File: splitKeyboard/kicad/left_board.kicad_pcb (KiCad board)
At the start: 2 copper layers, 305 x 136.1 mm, 131 parts

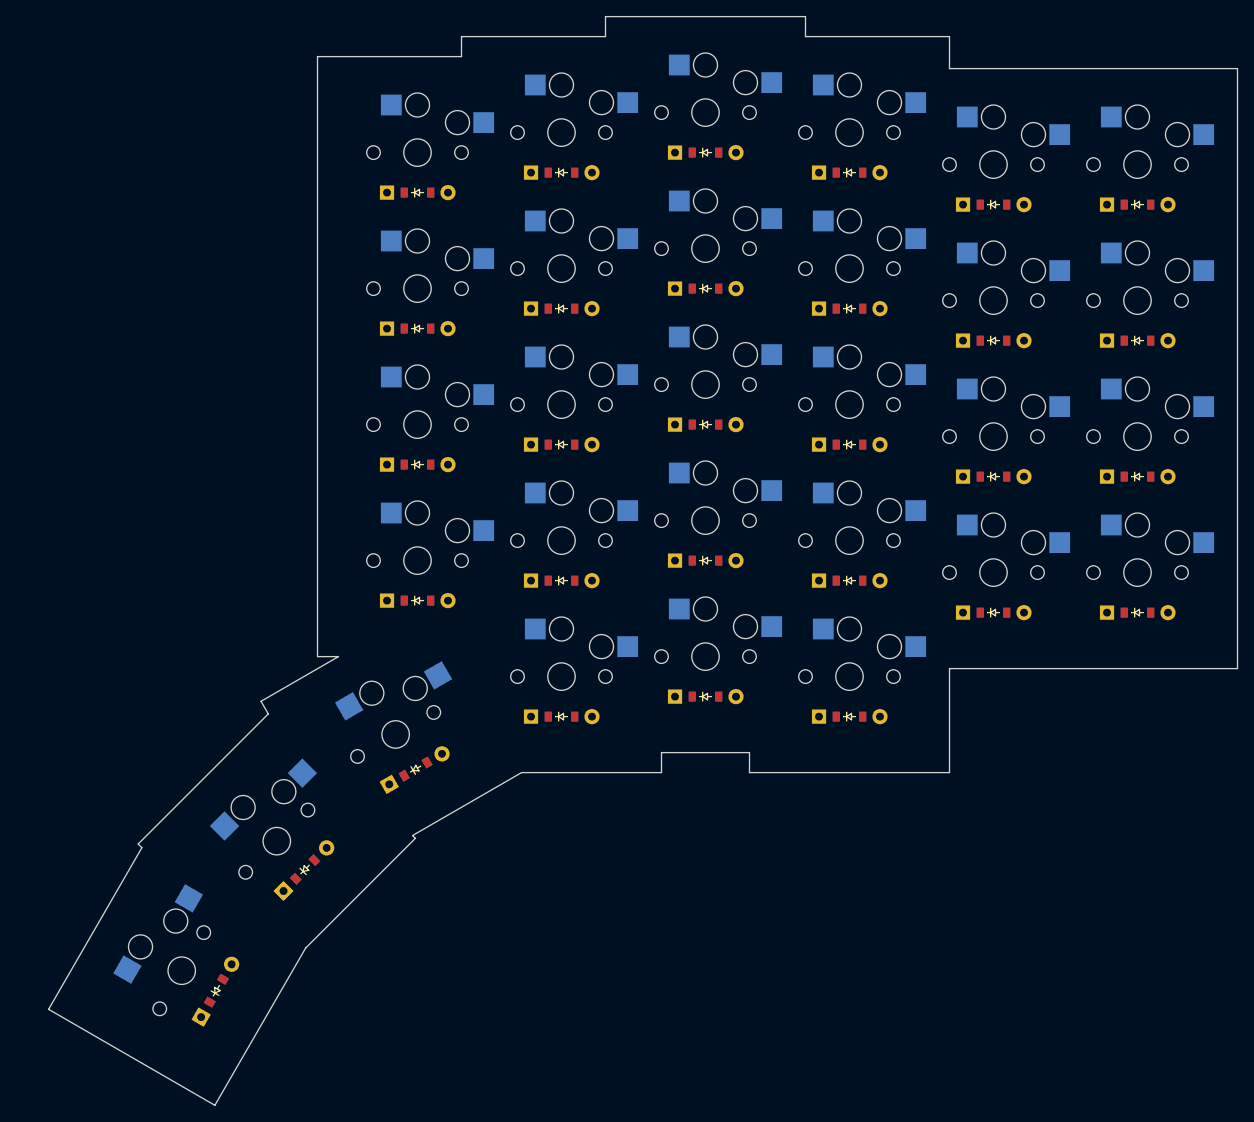
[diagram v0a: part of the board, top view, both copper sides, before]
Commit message: fix: got rid of unnecessary extra side
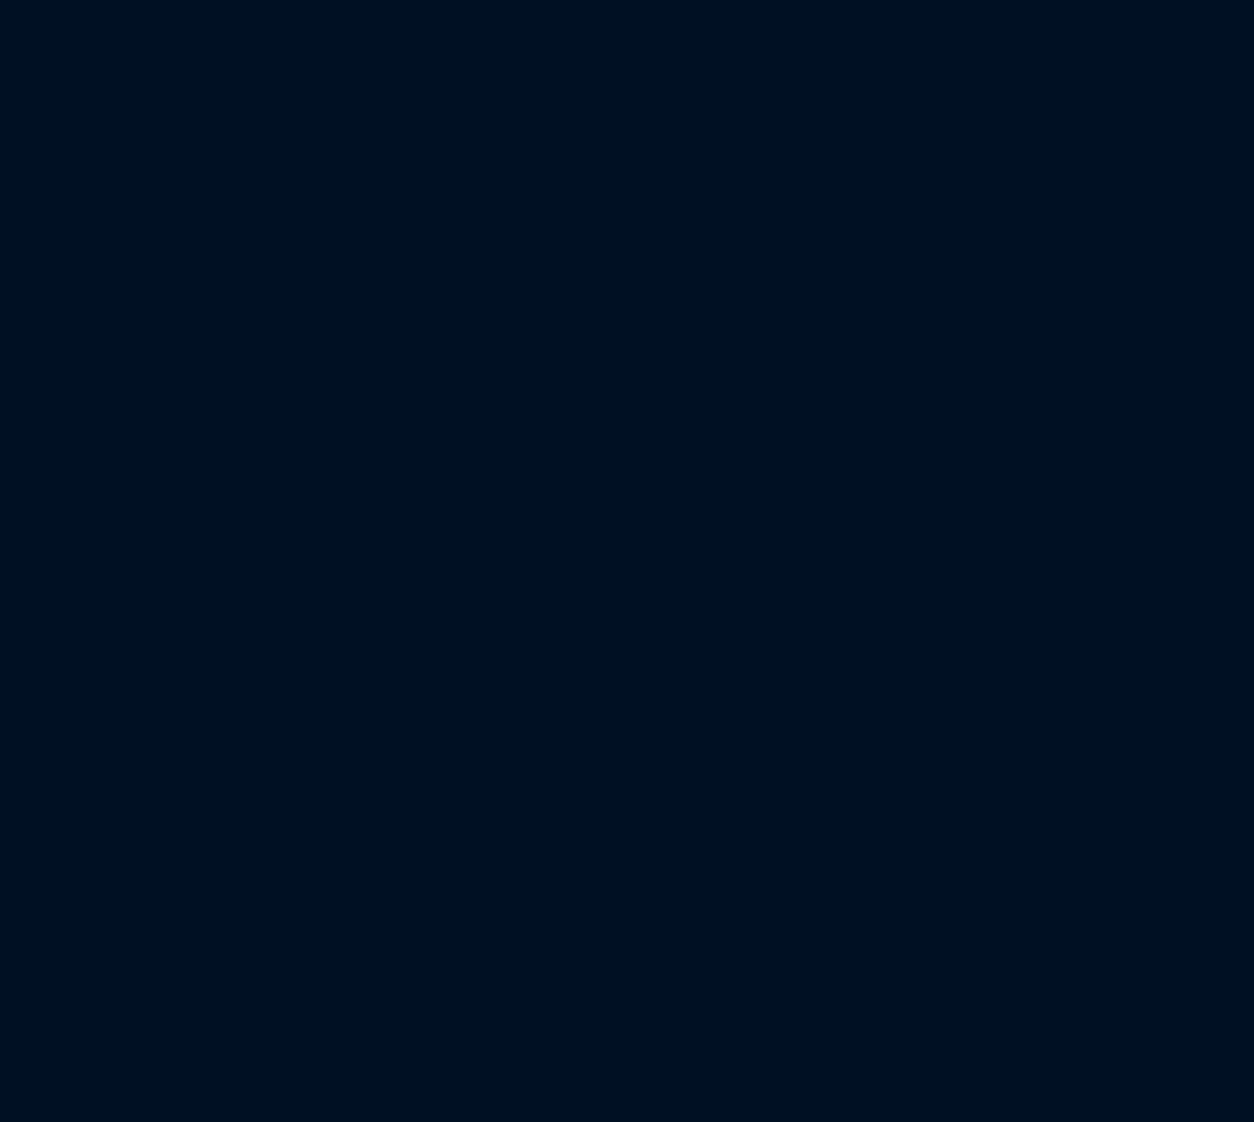
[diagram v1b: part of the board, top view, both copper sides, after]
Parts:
- removed D33, D34, D35, D36, D37, D38, D39, D40, D41, D42, D43, D44, D45, D46, D47, D48, D49, D50, D51, D52, D53, D54, D55, D56, D57, D58, D59, D60, D61, D62: , ComboDiode
- removed S31, S32, S33, S34, S35, S36, S37, S38, S39, S40, S41, S42, S43, S44, S45, S46, S47, S48, S49, S50, S51, S52, S53, S54, S55, S56, S57, S58, S59, S60: , PG1350
- moved D32 158.5 mm to (223.8, 44.5), turned to 90 degrees
- moved D31 158.3 mm to (227.8, 44.5), turned to 90 degrees
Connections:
- D31 pad 1: P7 -> GND
- D31 pad 2: mirror_outer_bottom -> P0
- D32 pad 1: P6 -> GND
- D32 pad 2: mirror_outer_home -> VCC
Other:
- board size 305 x 136.1 mm -> 148.6 x 136.1 mm
